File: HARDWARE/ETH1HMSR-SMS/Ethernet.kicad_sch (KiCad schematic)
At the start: 34 parts, among them J301 RJ45_Wuerth_7499010121A, U301 LAN8742A, Y301 NX5032GA-25

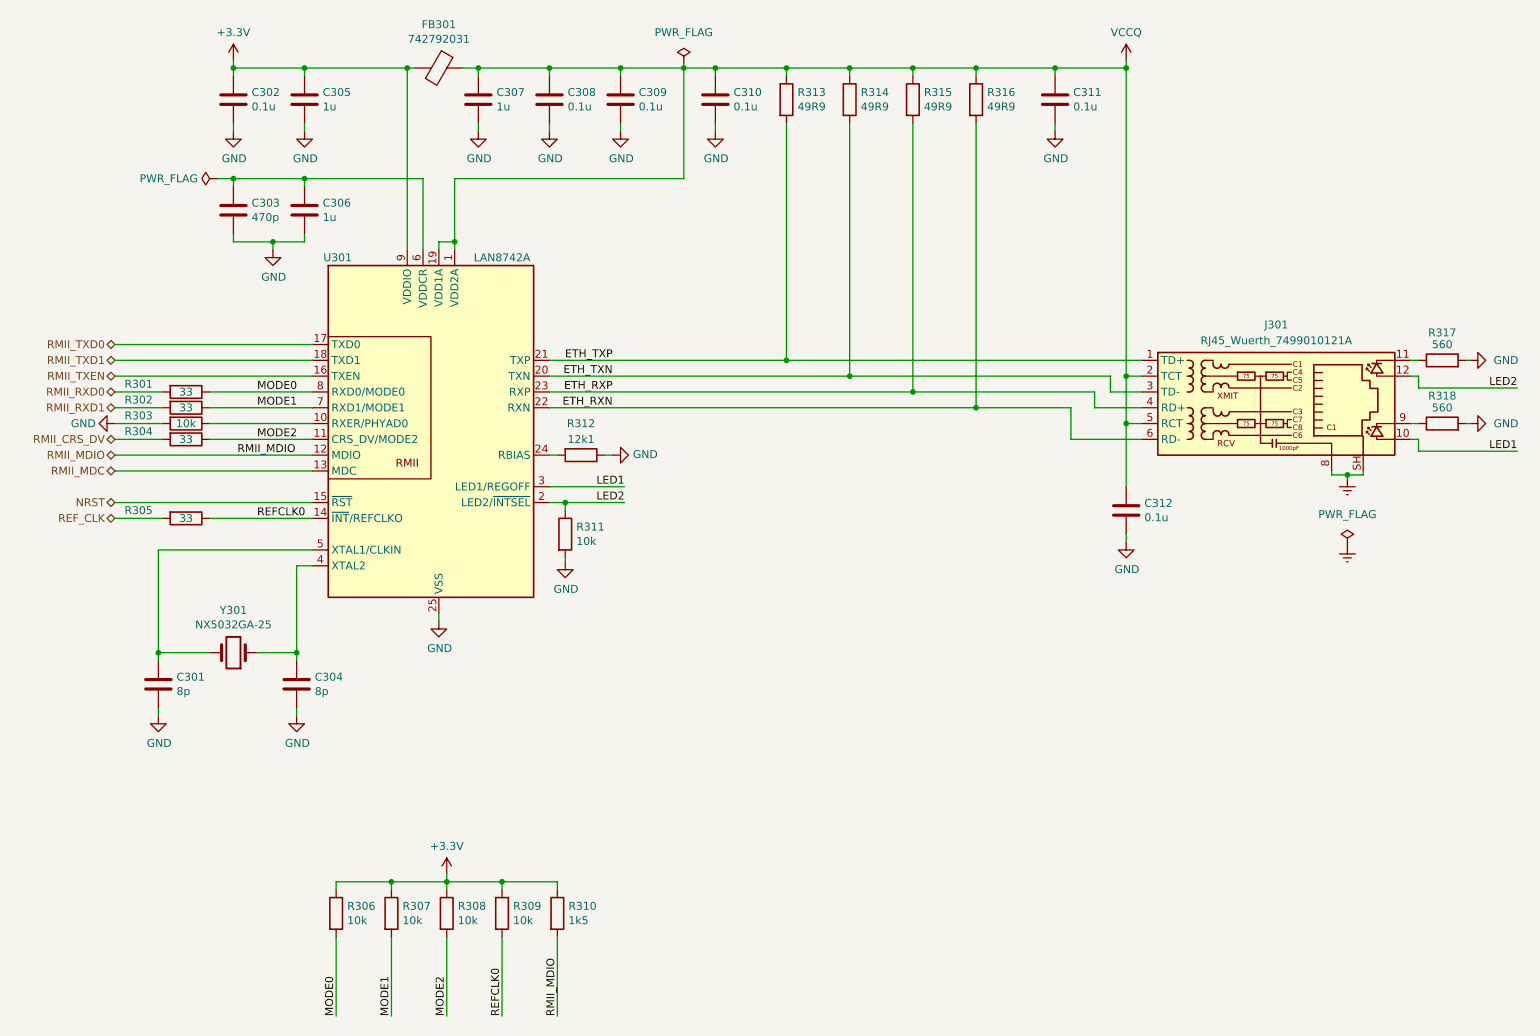
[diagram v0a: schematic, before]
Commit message: SW and HW development
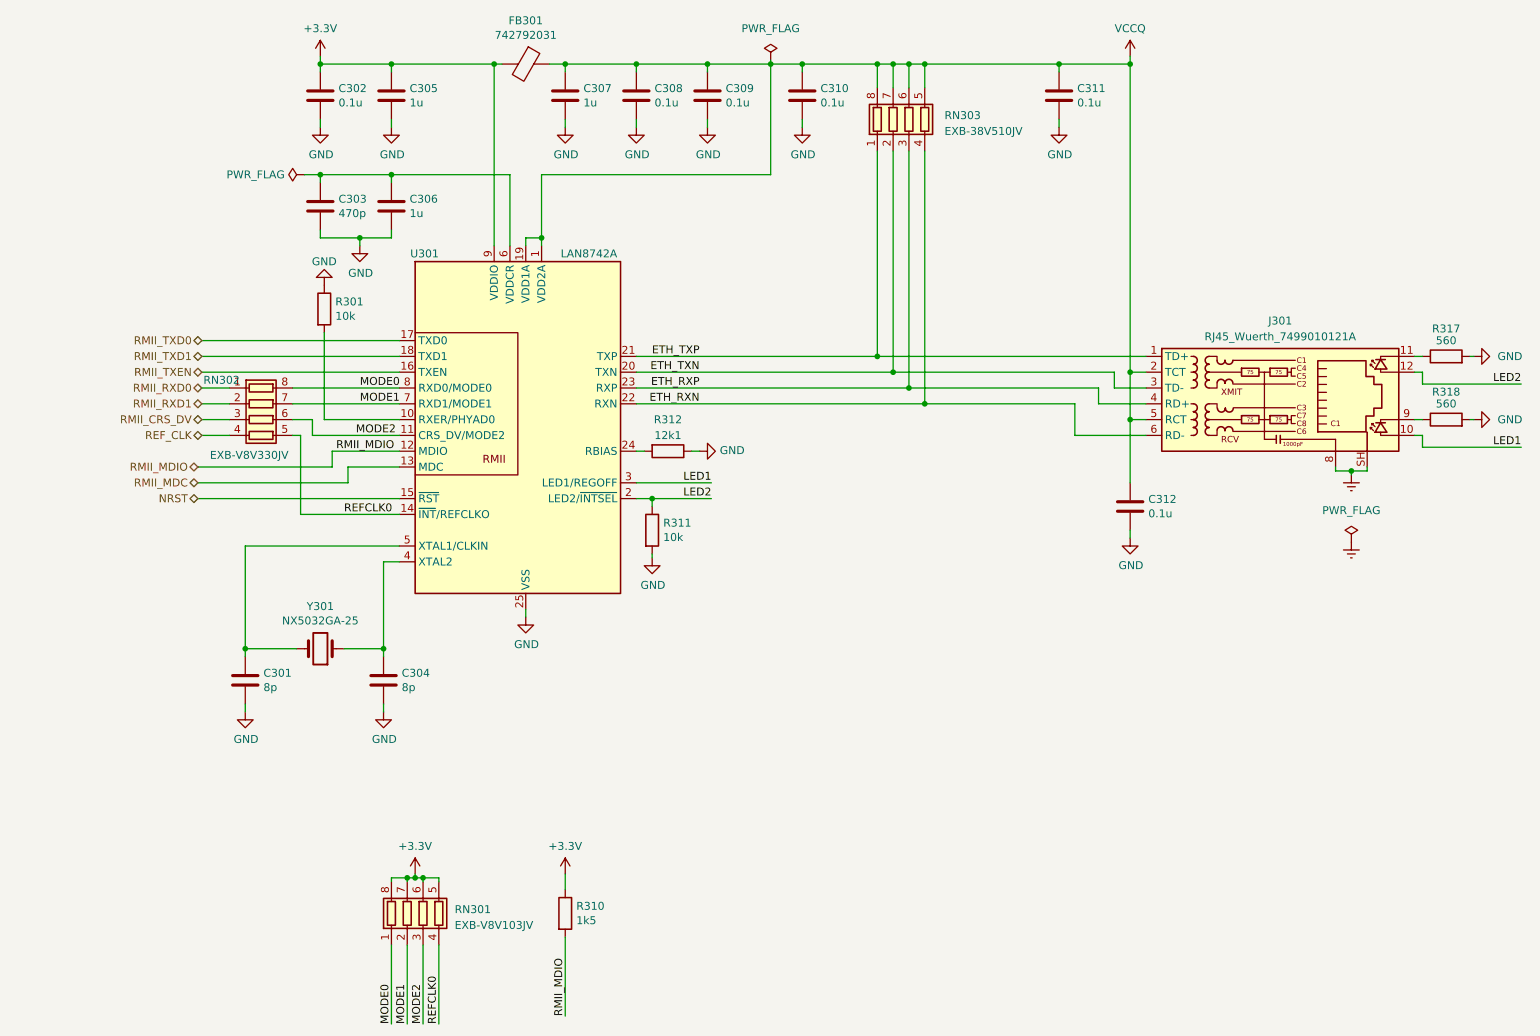
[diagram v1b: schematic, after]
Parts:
- removed R302, R304, R305: 33, Resistor_SMD:R_0603_1608Metric_Pad0.98x0.95mm_HandSolder, symbol Device:R
- removed R303, R306, R307, R308, R309: 10k, Resistor_SMD:R_0603_1608Metric_Pad0.98x0.95mm_HandSolder, symbol Device:R
- removed R313, R314, R315, R316: 49R9, Resistor_SMD:R_0603_1608Metric_Pad0.98x0.95mm_HandSolder, symbol Device:R
- added RN301: EXB-V8V103JV, Resistor_SMD:R_Array_Concave_4x0603, symbol Device:R_Pack04
- added RN302: EXB-V8V330JV, Resistor_SMD:R_Array_Concave_4x0603, symbol Device:R_Pack04
- added RN303: EXB-38V510JV, Resistor_SMD:R_Array_Concave_4x0603, symbol Device:R_Pack04
- R301: value 33 -> 10k
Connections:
- net +3.3V: now also RN301.5 (R4.2), RN301.6 (R3.2), RN301.7 (R2.2), RN301.8 (R1.2)
- net ETH_RXN: now also RN303.4 (R4.1)
- net ETH_RXP: now also RN303.3 (R3.1)
- net ETH_TXN: now also RN303.2 (R2.1)
- net ETH_TXP: now also RN303.1 (R1.1)
- net GND: now also R301.1
- net MODE0: now also RN301.1 (R1.1), RN302.8 (R1.2); no longer R301.1
- net MODE1: now also RN301.2 (R2.1), RN302.7 (R2.2)
- net MODE2: now also RN301.3 (R3.1), RN302.6 (R3.2)
- net REFCLK0: now also RN301.4 (R4.1), RN302.5 (R4.2)
- net REF_CLK: now also RN302.4 (R4.1)
- net RMII_CRS_DV: now also RN302.3 (R3.1)
- net RMII_RXD0: now also RN302.1 (R1.1); no longer R301.2
- net RMII_RXD1: now also RN302.2 (R2.1)
- net VCCQ: now also RN303.5 (R4.2), RN303.6 (R3.2), RN303.7 (R2.2), RN303.8 (R1.2)
- net at U301.10 (RXER/PHYAD0): now also R301.2
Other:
- moved on the sheet: C301, C302, C303, C304, C305, C306, C307, C308, C309, C310, C311, C312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
